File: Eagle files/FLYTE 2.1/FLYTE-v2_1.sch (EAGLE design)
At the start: 68 parts, among them Q1 IRF540NPBF, Q2 IRF540NPBF, U3 ADS1115IDGSR, U4 H3LIS200DLTR, U6 W25Q32JVSSIQ

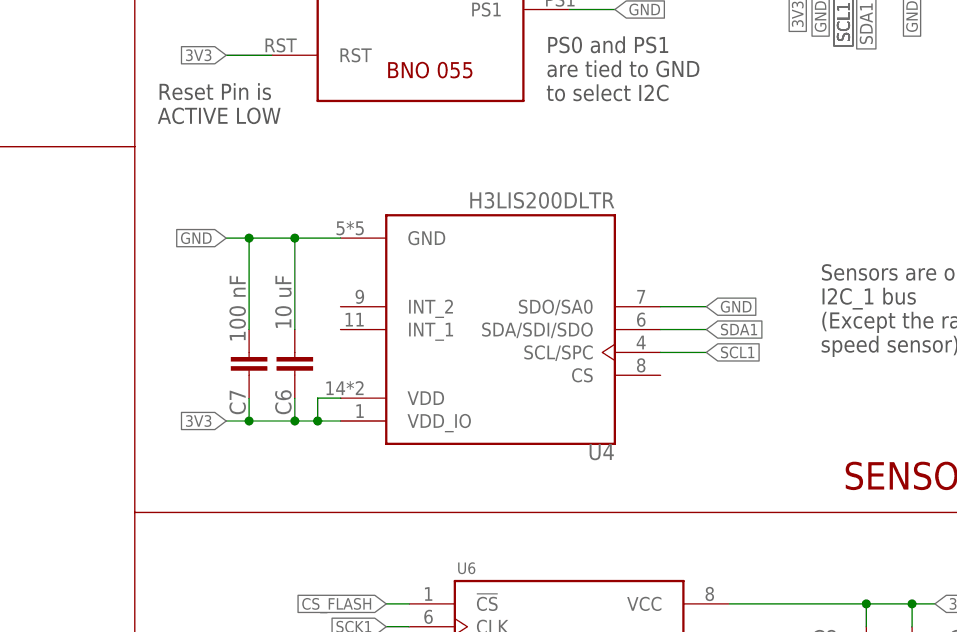
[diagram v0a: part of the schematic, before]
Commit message: motor controller re design
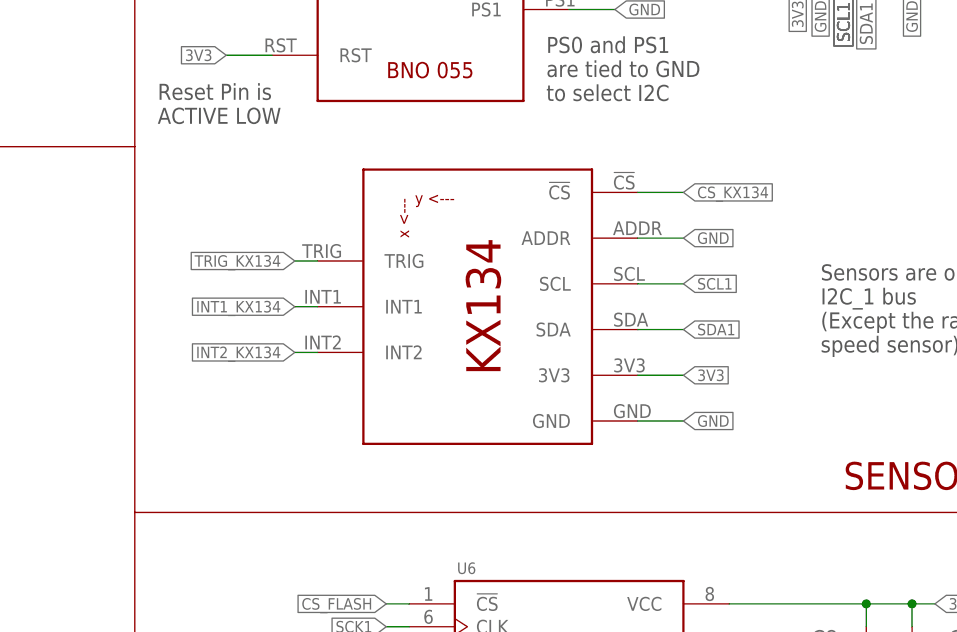
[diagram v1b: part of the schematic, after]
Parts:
- removed C6: 10 uF, SparkFun-Capacitors:22UF-0805-6.3V-20%
- removed C7: 100 nF, SparkFun-Capacitors:22UF-0805-6.3V-20%
- removed U4: H3LIS200DLTR, H3LIS200DLTR:H3LIS200DLTR
- added U$2: KX134-BREAKOUT, KX134_Breakout:KX134-BREAKOUT
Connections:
- new net CS_KX134: U$2.!CS
- new net INT1_KX134: U$2.INT1
- new net INT2_KX134: U$2.INT2
- new net TRIG_KX134: U$2.TRIG
- net 3V3: now also U$2.3V3; no longer C6.1, C7.1, U4.VDD, U4.VDD_IO
- net GND: now also U$2.ADDR, U$2.GND; no longer C6.2, C7.2, U4.GND, U4.SDO/SA0
- net SCL1: now also U$2.SCL; no longer U4.SCL/SPC
- net SDA1: now also U$2.SDA; no longer U4.SDA/SDI/SDO
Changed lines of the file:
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@@
 <part name="C5" library="SparkFun-Capacitors" deviceset="22UF" device="-0805-6.3V-20%" override_package3d_urn="urn:adsk.eagle:package:40331879/2" override_package_urn="urn:adsk.eagle:footprint:40331880/1" value="100 nF"/>
 <part name="U$4" library="BNO055" deviceset="BNO055" device="" override_package3d_urn="urn:adsk.eagle:package:43006369/2" override_package_urn="urn:adsk.eagle:footprint:43006370/1"/>
-<part name="U4" library="H3LIS200DLTR" deviceset="H3LIS200DLTR" device="" override_package3d_urn="urn:adsk.eagle:package:43006487/2" override_package_urn="urn:adsk.eagle:footprint:43006488/1"/>
-<part name="C6" library="SparkFun-Capacitors" deviceset="22UF" device="-0805-6.3V-20%" override_package3d_urn="urn:adsk.eagle:package:40331879/2" override_package_urn="urn:adsk.eagle:footprint:40331880/1" value="10 uF"/>
-<part name="C7" library="SparkFun-Capacitors" deviceset="22UF" device="-0805-6.3V-20%" override_package3d_urn="urn:adsk.eagle:package:40331879/2" override_package_urn="urn:adsk.eagle:footprint:40331880/1" value="100 nF"/>
 <part name="R2" library="rcl" library_urn="urn:adsk.eagle:library:334" deviceset="R-US_" device="R0805" package3d_urn="urn:adsk.eagle:package:23553/2" value="4.7K ohm"/>
 <part name="R5" library="rcl" library_urn="urn:adsk.eagle:library:334" deviceset="R-US_" device="R0805" package3d_urn="urn:adsk.eagle:package:23553/2" value="4.7K ohm"/>
@@
 <part name="INTERFACE" library="TS04-66-95-BK-100-SMT" deviceset="TS04-66-95-BK-100-SMT" device=""/>
 <part name="R15" library="rcl" library_urn="urn:adsk.eagle:library:334" deviceset="R-US_" device="R0805" package3d_urn="urn:adsk.eagle:package:23553/2" value="4.7K ohm"/>
+<part name="U$2" library="KX134_Breakout" deviceset="KX134-BREAKOUT" device=""/>
 </parts>
 <sheets>
@@
 </instance>
 <instance part="U$4" gate="G$1" x="320.04" y="157.48" smashed="yes" rot="R270"/>
-<instance part="U4" gate="G$1" x="340.36" y="106.68" smashed="yes" rot="R180">
-<attribute name="NAME" x="353.0693" y="93.9707" size="1.779309375" layer="95" rot="R180"/>
-<attribute name="VALUE" x="353.0645" y="121.9254" size="1.77863125" layer="96" rot="R180"/>
-</instance>
-<instance part="C6" gate="G$1" x="317.5" y="104.14" smashed="yes" rot="R180">
-<attribute name="NAME" x="315.341" y="100.076" size="1.778" layer="95" font="vector" rot="R270"/>
-<attribute name="VALUE" x="315.341" y="112.776" size="1.778" layer="96" font="vector" rot="R270"/>
-</instance>
-<instance part="C7" gate="G$1" x="312.42" y="104.14" smashed="yes" rot="R180">
-<attribute name="NAME" x="310.261" y="100.076" size="1.778" layer="95" font="vector" rot="R270"/>
-<attribute name="VALUE" x="310.261" y="112.776" size="1.778" layer="96" font="vector" rot="R270"/>
-</instance>
 <instance part="R2" gate="G$1" x="109.22" y="22.86" smashed="yes" rot="R180">
 <attribute name="NAME" x="115.57" y="21.3614" size="1.778" layer="95" rot="R180"/>
@@
 <attribute name="VALUE" x="135.89" y="34.798" size="1.778" layer="96"/>
 </instance>
+<instance part="U$2" gate="A" x="350.52" y="96.52" smashed="yes" rot="R90"/>
 </instances>
 <busses>
@@
 <wire x1="332.74" y1="220.98" x2="327.66" y2="220.98" width="0.1524" layer="91"/>
 <label x="327.66" y="220.98" size="1.27" layer="95" rot="R180" xref="yes"/>
-</segment>
-<segment>
-<pinref part="U4" gate="G$1" pin="GND"/>
-<wire x1="322.58" y1="116.84" x2="317.5" y2="116.84" width="0.1524" layer="91"/>
-<label x="309.88" y="116.84" size="1.27" layer="95" rot="R180" xref="yes"/>
-<pinref part="C6" gate="G$1" pin="2"/>
-<wire x1="317.5" y1="116.84" x2="312.42" y2="116.84" width="0.1524" layer="91"/>
-<wire x1="312.42" y1="116.84" x2="309.88" y2="116.84" width="0.1524" layer="91"/>
-<wire x1="317.5" y1="106.68" x2="317.5" y2="116.84" width="0.1524" layer="91"/>
-<junction x="317.5" y="116.84"/>
-<pinref part="C7" gate="G$1" pin="2"/>
-<wire x1="312.42" y1="106.68" x2="312.42" y2="116.84" width="0.1524" layer="91"/>
-<junction x="312.42" y="116.84"/>
-</segment>
-<segment>
-<pinref part="U4" gate="G$1" pin="SDO/SA0"/>
-<wire x1="358.14" y1="109.22" x2="363.22" y2="109.22" width="0.1524" layer="91"/>
-<label x="363.22" y="109.22" size="1.27" layer="95" xref="yes"/>
 </segment>
 <segment>
@@
 <label x="386.08" y="63.5" size="1.27" layer="95" rot="R270" xref="yes"/>
 </segment>
+<segment>
+<pinref part="U$2" gate="A" pin="ADDR"/>
+<wire x1="355.6" y1="116.84" x2="360.68" y2="116.84" width="0.1524" layer="91"/>
+<label x="360.68" y="116.84" size="1.27" layer="95" xref="yes"/>
+</segment>
+<segment>
+<pinref part="U$2" gate="A" pin="GND"/>
+<wire x1="355.6" y1="96.52" x2="360.68" y2="96.52" width="0.1524" layer="91"/>
+<label x="360.68" y="96.52" size="1.27" layer="95" xref="yes"/>
+</segment>
 </net>
 <net name="VCC" class="0">
@@
 </segment>
 <segment>
-<pinref part="U4" gate="G$1" pin="SCL/SPC"/>
-<wire x1="358.14" y1="104.14" x2="363.22" y2="104.14" width="0.1524" layer="91"/>
-<label x="363.22" y="104.14" size="1.27" layer="95" xref="yes"/>
+<pinref part="U$2" gate="A" pin="SCL"/>
+<wire x1="355.6" y1="111.76" x2="360.68" y2="111.76" width="0.1524" layer="91"/>
+<label x="360.68" y="111.76" size="1.27" layer="95" xref="yes"/>
 </segment>
 </net>
@@
 </segment>
 <segment>
-<pinref part="U4" gate="G$1" pin="VDD_IO"/>
-<wire x1="322.58" y1="96.52" x2="320.04" y2="96.52" width="0.1524" layer="91"/>
-<label x="309.88" y="96.52" size="1.27" layer="95" rot="R180" xref="yes"/>
-<pinref part="U4" gate="G$1" pin="VDD"/>
-<wire x1="320.04" y1="96.52" x2="317.5" y2="96.52" width="0.1524" layer="91"/>
-<wire x1="317.5" y1="96.52" x2="312.42" y2="96.52" width="0.1524" layer="91"/>
-<wire x1="312.42" y1="96.52" x2="309.88" y2="96.52" width="0.1524" layer="91"/>
-<wire x1="322.58" y1="99.06" x2="320.04" y2="99.06" width="0.1524" layer="91"/>
-<wire x1="320.04" y1="99.06" x2="320.04" y2="96.52" width="0.1524" layer="91"/>
-<junction x="320.04" y="96.52"/>
-<pinref part="C6" gate="G$1" pin="1"/>
-<wire x1="317.5" y1="96.52" x2="317.5" y2="99.06" width="0.1524" layer="91"/>
-<junction x="317.5" y="96.52"/>
-<pinref part="C7" gate="G$1" pin="1"/>
-<wire x1="312.42" y1="96.52" x2="312.42" y2="99.06" width="0.1524" layer="91"/>
-<junction x="312.42" y="96.52"/>
-</segment>
-<segment>
 <wire x1="114.3" y1="22.86" x2="116.84" y2="22.86" width="0.1524" layer="91"/>
 <label x="116.84" y="22.86" size="1.27" layer="95" xref="yes"/>
@@
 <wire x1="134.62" y1="38.1" x2="132.08" y2="38.1" width="0.1524" layer="91"/>
 <label x="132.08" y="38.1" size="1.27" layer="95" rot="R180" xref="yes"/>
+</segment>
+<segment>
+<pinref part="U$2" gate="A" pin="3V3"/>
+<wire x1="355.6" y1="101.6" x2="360.68" y2="101.6" width="0.1524" layer="91"/>
+<label x="360.68" y="101.6" size="1.27" layer="95" xref="yes"/>
 </segment>
 </net>
@@
 </segment>
 <segment>
-<pinref part="U4" gate="G$1" pin="SDA/SDI/SDO"/>
-<wire x1="358.14" y1="106.68" x2="363.22" y2="106.68" width="0.1524" layer="91"/>
-<label x="363.22" y="106.68" size="1.27" layer="95" xref="yes"/>
+<pinref part="U$2" gate="A" pin="SDA"/>
+<wire x1="355.6" y1="106.68" x2="360.68" y2="106.68" width="0.1524" layer="91"/>
+<label x="360.68" y="106.68" size="1.27" layer="95" xref="yes"/>
 </segment>
 </net>
@@
 </segment>
 </net>
+<net name="CS_KX134" class="0">
+<segment>
+<pinref part="U$2" gate="A" pin="!CS"/>
+<wire x1="355.6" y1="121.92" x2="360.68" y2="121.92" width="0.1524" layer="91"/>
+<label x="360.68" y="121.92" size="1.27" layer="95" xref="yes"/>
+</segment>
+</net>
+<net name="TRIG_KX134" class="0">
+<segment>
+<pinref part="U$2" gate="A" pin="TRIG"/>
+<wire x1="320.04" y1="114.3" x2="317.5" y2="114.3" width="0.1524" layer="91"/>
+<label x="317.5" y="114.3" size="1.27" layer="95" rot="R180" xref="yes"/>
+</segment>
+</net>
+<net name="INT1_KX134" class="0">
+<segment>
+<pinref part="U$2" gate="A" pin="INT1"/>
+<wire x1="320.04" y1="109.22" x2="317.5" y2="109.22" width="0.1524" layer="91"/>
+<label x="317.5" y="109.22" size="1.27" layer="95" rot="R180" xref="yes"/>
+</segment>
+</net>
+<net name="INT2_KX134" class="0">
+<segment>
+<pinref part="U$2" gate="A" pin="INT2"/>
+<wire x1="320.04" y1="104.14" x2="317.5" y2="104.14" width="0.1524" layer="91"/>
+<label x="317.5" y="104.14" size="1.27" layer="95" rot="R180" xref="yes"/>
+</segment>
+</net>
